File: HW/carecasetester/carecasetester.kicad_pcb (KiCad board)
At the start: 2 copper layers, 158.3 x 161.1 mm, 86 parts, among them J1 Conn_01x16_Female, J10-TP22 Conn_01x01_Male, J11-TP7 Conn_01x01_Male, J12-TP14 Conn_01x01_Male, J13-TP23 Conn_01x01_Male, J14-TP17 Conn_01x01_Male, J15 Conn_01x16_Male, J15-TP1 Conn_01x01_Male, J15-TP20 Conn_01x01_Male, J16-TP2 Conn_01x01_Male, J16-TP24 Conn_01x01_Male, J17-TP3 Conn_01x01_Male, J18-TP4 Conn_01x01_Male, J19-TP6 Conn_01x01_Male, J2 Conn_01x16_Female, J20-TP9 Conn_01x01_Male, J21-TP10 Conn_01x01_Male, J22-TP11 Conn_01x01_Male, J23-TP12 Conn_01x01_Male, J24-TP15 Conn_01x01_Male, J25-TP18 Conn_01x01_Male, J26-TP5 Conn_01x01_Male, J27-TP26 Conn_01x01_Male, J28-TP25 Conn_01x01_Male, J3 Conn_01x04_Female, J4 Conn_01x06_Male, J4-TP16 Conn_01x01_Male, J5 12V_Psu, J5-TP8 Conn_01x01_Male, J5-~E1 Conn_01x02_Male, J6-TP21 Conn_01x01_Male, J7-TP27 Conn_01x01_Male, J8-TP13 Conn_01x01_Male, J9-TP19 Conn_01x01_Male, K1 AZ952, K2 AZ952, Q1 BC847W, Q2 BC847W, SW1 SW_DIP_x02, U1 CD74HC4067M, U2 L7805

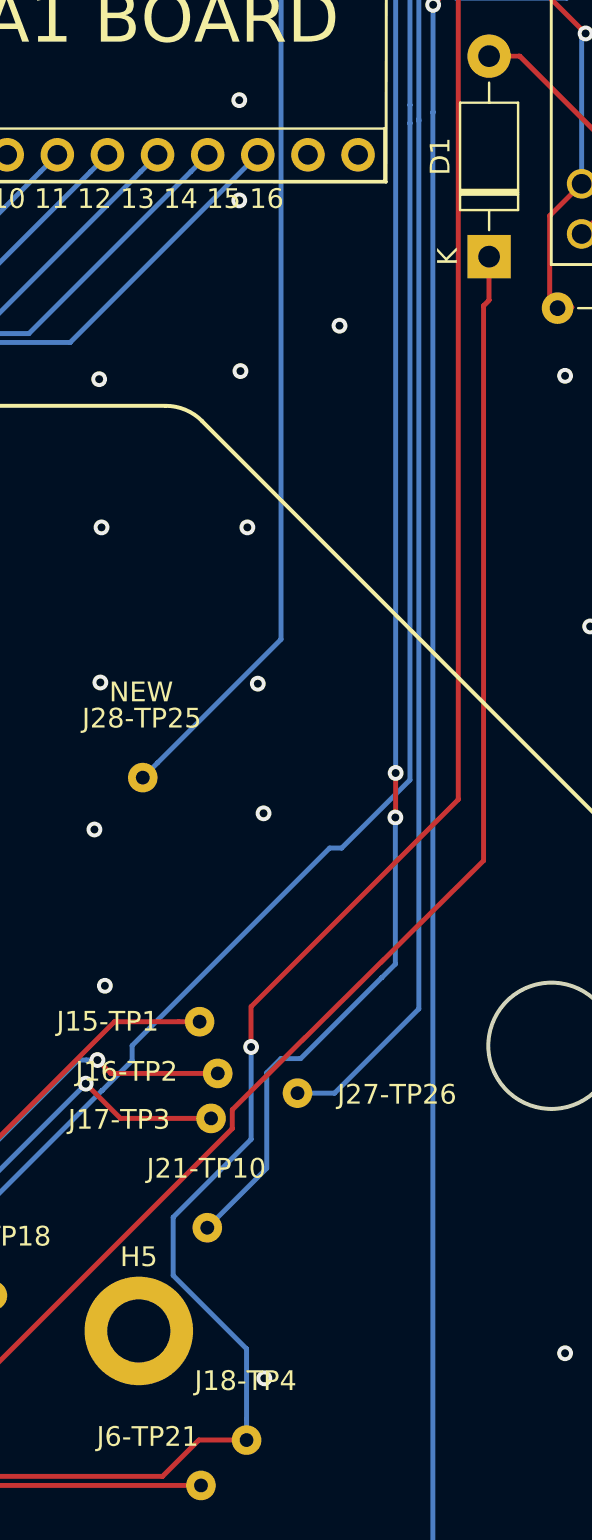
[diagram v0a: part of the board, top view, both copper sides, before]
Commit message: dfgdfg
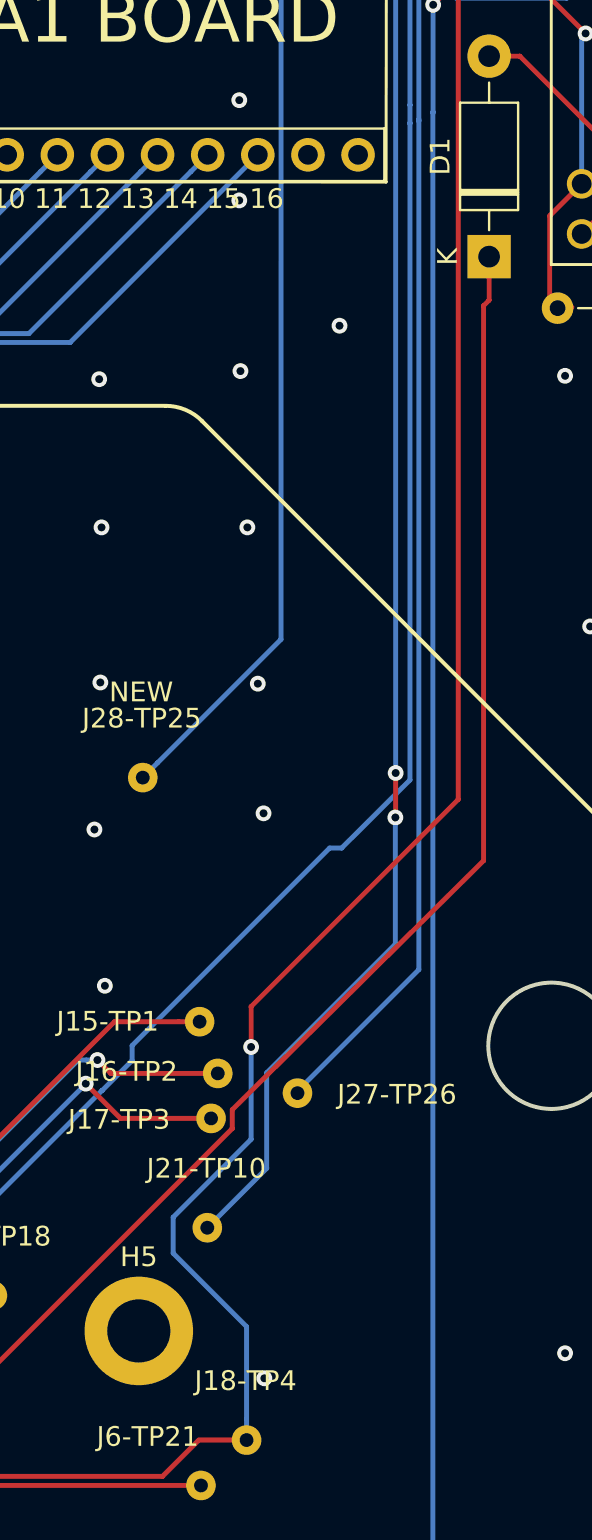
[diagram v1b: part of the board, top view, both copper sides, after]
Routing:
- net Net-(J15-Pad14): track 159.0 -> 157.9 mm
- net Net-(J15-Pad8): track 179.8 -> 179.2 mm
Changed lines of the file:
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@@
     (thickness 1)
     (drawings 156)
-    (tracks 1314)
+    (tracks 1310)
     (zones 0)
     (modules 86)
@@
   (segment (start 183.83002 33.43) (end 183.61001 33.65001) (width 0.25) (layer B.Cu) (net 29))
   (segment (start 205.29 37.3) (end 205.29 37.29) (width 0.25) (layer B.Cu) (net 29))
-  (segment (start 204.21999 99.85) (end 208.49 95.57999) (width 0.25) (layer B.Cu) (net 29))
-  (segment (start 202.34 99.85) (end 204.21999 99.85) (width 0.25) (layer B.Cu) (net 29))
   (segment (start 208.49 40.49) (end 206.550001 38.550001) (width 0.25) (layer B.Cu) (net 29))
   (segment (start 208.49 40.49) (end 208.49 50.58) (width 0.25) (layer B.Cu) (net 29))
-  (segment (start 208.49 95.57999) (end 208.49 50.58) (width 0.25) (layer B.Cu) (net 29))
   (segment (start 208.49 50.58) (end 208.49 50.49) (width 0.25) (layer B.Cu) (net 29))
+  (segment (start 208.49 93.59) (end 208.49 50.58) (width 0.25) (layer B.Cu) (net 29))
+  (segment (start 202.34 99.85) (end 202.34 99.74) (width 0.25) (layer B.Cu) (net 29))
+  (segment (start 202.34 99.74) (end 208.49 93.59) (width 0.25) (layer B.Cu) (net 29))
   (via (at 141.64 84.48) (size 0.8) (drill 0.4) (layers F.Cu B.Cu) (net 30))
   (segment (start 141.64 84.48) (end 142.52 85.36) (width 0.25) (layer F.Cu) (net 30))
@@
   (segment (start 207.31499 83.626846) (end 207.31499 85.86501) (width 0.25) (layer F.Cu) (net 33))
   (segment (start 207.31499 85.86501) (end 207.3 85.88) (width 0.25) (layer F.Cu) (net 33))
-  (segment (start 200.78 98.82) (end 200.78 103.66) (width 0.25) (layer B.Cu) (net 33))
-  (segment (start 201.5 98.1) (end 200.78 98.82) (width 0.25) (layer B.Cu) (net 33))
-  (segment (start 200.78 103.66) (end 197.77 106.67) (width 0.25) (layer B.Cu) (net 33))
-  (segment (start 207.3 85.88) (end 207.3 93.31) (width 0.25) (layer B.Cu) (net 33))
-  (segment (start 207.3 93.31) (end 206.62 93.99) (width 0.25) (layer B.Cu) (net 33))
-  (segment (start 206.608998 93.99) (end 202.498998 98.1) (width 0.25) (layer B.Cu) (net 33))
-  (segment (start 202.498998 98.1) (end 201.5 98.1) (width 0.25) (layer B.Cu) (net 33))
-  (segment (start 206.62 93.99) (end 206.608998 93.99) (width 0.25) (layer B.Cu) (net 33))
   (segment (start 201.04 34.96) (end 181.74 34.96) (width 0.25) (layer B.Cu) (net 33))
   (segment (start 201.46 34.96) (end 201.04 34.96) (width 0.25) (layer B.Cu) (net 33))
@@
   (segment (start 181.12 35.58) (end 181.74 34.96) (width 0.25) (layer F.Cu) (net 33))
   (segment (start 137.260064 36.579936) (end 138.79 35.05) (width 0.25) (layer B.Cu) (net 33))
+  (segment (start 200.78 98.82) (end 200.78 103.66) (width 0.25) (layer B.Cu) (net 33))
+  (segment (start 200.78 103.66) (end 197.77 106.67) (width 0.25) (layer B.Cu) (net 33))
+  (segment (start 207.3 85.88) (end 207.3 92.3) (width 0.25) (layer B.Cu) (net 33))
+  (segment (start 207.3 92.3) (end 200.78 98.82) (width 0.25) (layer B.Cu) (net 33))
   (via (at 150.46 84.47) (size 0.8) (drill 0.4) (layers F.Cu B.Cu) (net 34))
   (segment (start 150.46 84.47) (end 156.57 84.47) (width 0.25) (layer F.Cu) (net 34))
@@
   (via (at 199.99 97.51) (size 0.8) (drill 0.4) (layers F.Cu B.Cu) (net 67))
   (segment (start 199.99 95.463002) (end 199.99 97.51) (width 0.25) (layer F.Cu) (net 67))
-  (segment (start 199.99 97.51) (end 199.99 102.19) (width 0.25) (layer B.Cu) (net 67))
-  (segment (start 199.99 102.19) (end 196.04 106.14) (width 0.25) (layer B.Cu) (net 67))
-  (segment (start 199.76 116.36934) (end 199.76 117.43) (width 0.25) (layer B.Cu) (net 67))
-  (segment (start 199.76 112.808998) (end 199.76 116.36934) (width 0.25) (layer B.Cu) (net 67))
-  (segment (start 196.04 109.088998) (end 199.76 112.808998) (width 0.25) (layer B.Cu) (net 67))
-  (segment (start 196.04 106.14) (end 196.04 109.088998) (width 0.25) (layer B.Cu) (net 67))
   (segment (start 197.34 117.43) (end 199.76 117.43) (width 0.25) (layer F.Cu) (net 67))
   (segment (start 195.5 119.27) (end 197.34 117.43) (width 0.25) (layer F.Cu) (net 67))
+  (segment (start 199.76 116.36934) (end 199.76 117.43) (width 0.25) (layer B.Cu) (net 67))
+  (segment (start 199.99 97.51) (end 199.99 102.19) (width 0.25) (layer B.Cu) (net 67))
+  (segment (start 196.04 106.14) (end 196.04 107.96) (width 0.25) (layer B.Cu) (net 67))
+  (segment (start 199.99 102.19) (end 196.04 106.14) (width 0.25) (layer B.Cu) (net 67))
+  (segment (start 196.04 107.96) (end 199.76 111.68) (width 0.25) (layer B.Cu) (net 67))
+  (segment (start 199.76 111.68) (end 199.76 116.36934) (width 0.25) (layer B.Cu) (net 67))
   (segment (start 140.95 19.617919) (end 141.927919 18.64) (width 0.25) (layer F.Cu) (net 68))
   (segment (start 140.95 20.82) (end 140.95 19.617919) (width 0.25) (layer F.Cu) (net 68))
